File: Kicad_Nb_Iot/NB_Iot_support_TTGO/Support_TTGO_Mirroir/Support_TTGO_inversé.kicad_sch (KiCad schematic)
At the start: 12 parts, among them J1 Conn_01x10, J10 Conn_01x02, J11 Conn_01x02, J2 Conn_01x10, J3 Conn_01x04, J4 Conn_01x04, J5 Conn_01x04, J7 Conn_01x03, J8 Conn_01x04, J9 Conn_01x02, Q1 PMBT2222A,215

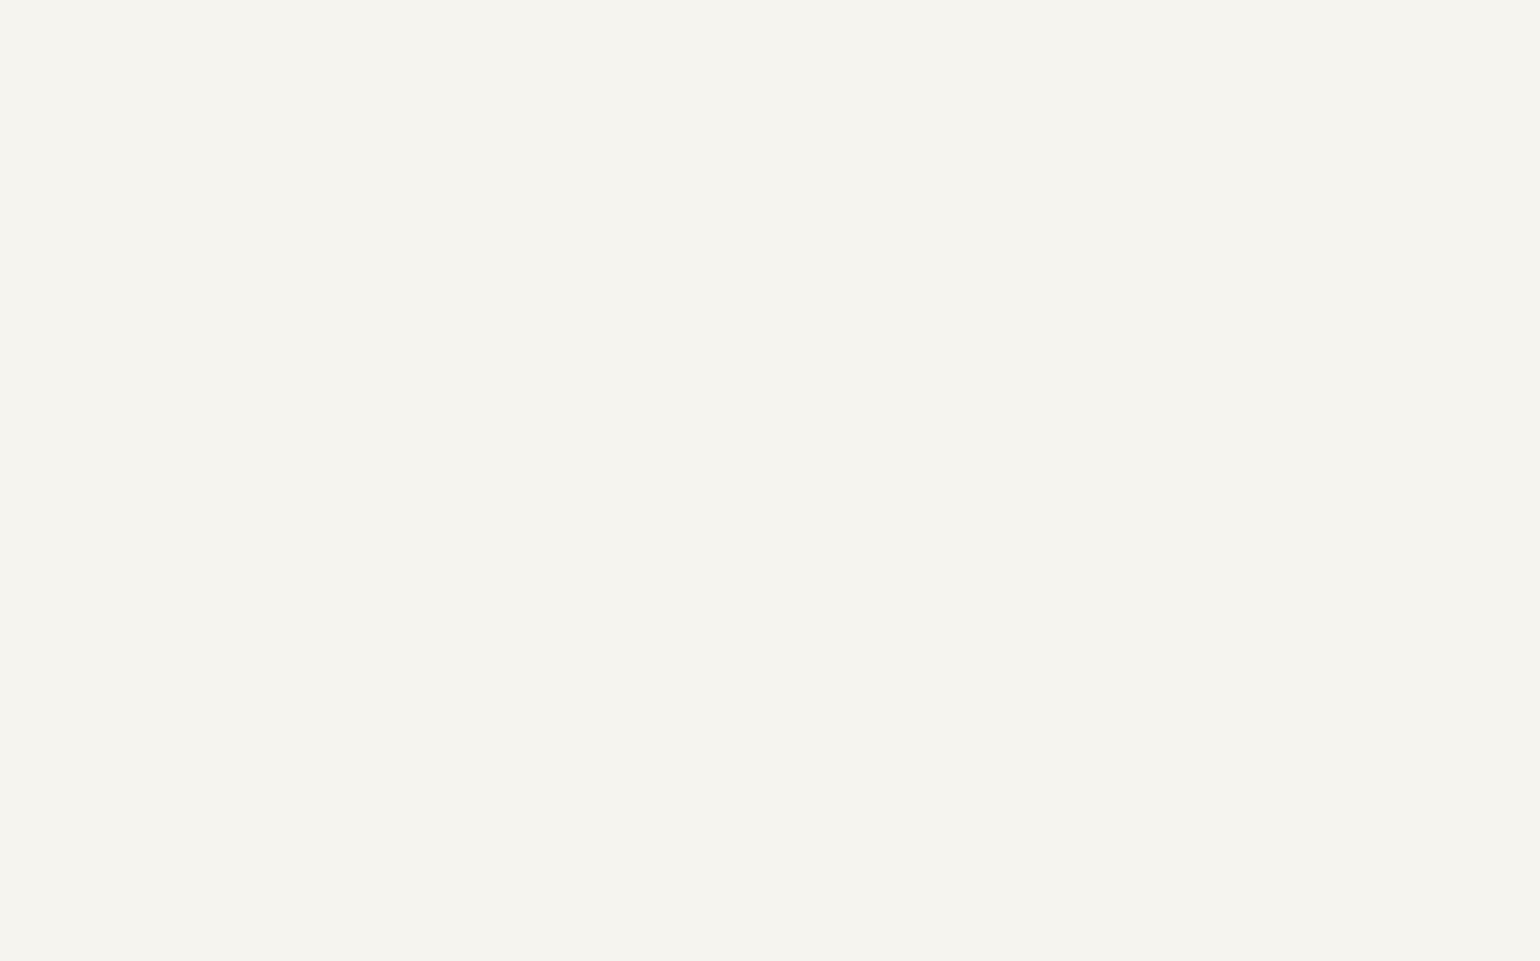
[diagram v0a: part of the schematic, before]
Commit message: update
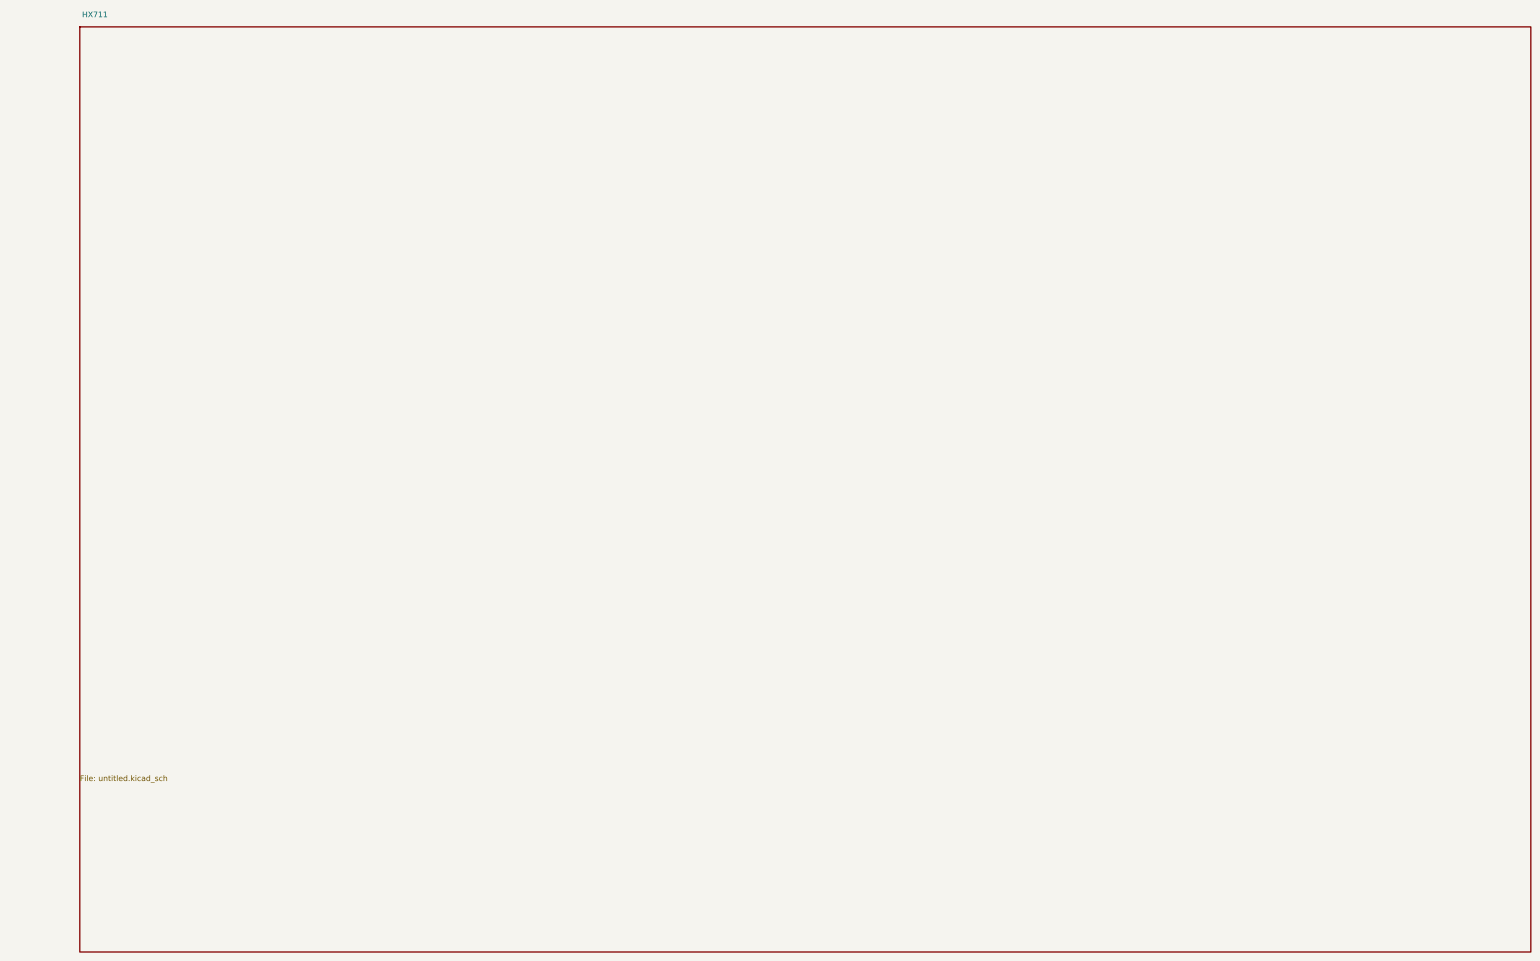
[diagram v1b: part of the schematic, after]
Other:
- added sheet HX711 (untitled.kicad_sch)
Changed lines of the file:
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@@
+    )
+  )
+  (sheet (at 312.42 0.508) (size 328.676 209.55)
+    (stroke (width 0.1524) (type solid))
+    (fill (color 0 0 0 0.0000))
+    (property "Sheetname" "HX711" (at 312.928 -1.524 0)
+      (effects (font (size 1.27 1.27)) (justify left bottom))
+    )
+    (property "Sheetfile" "untitled.kicad_sch" (at 312.42 170.0026 0)
+      (effects (font (size 1.27 1.27)) (justify left top))
+    )
+    (instances
+      (project "Support_TTGO_inversé"
+        (path "/ec613b36-6881-4eb0-a769-baf137e1cac3" (page "2"))
+      )
     )
   )
